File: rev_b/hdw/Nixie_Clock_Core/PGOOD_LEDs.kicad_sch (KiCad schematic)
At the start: 17 parts

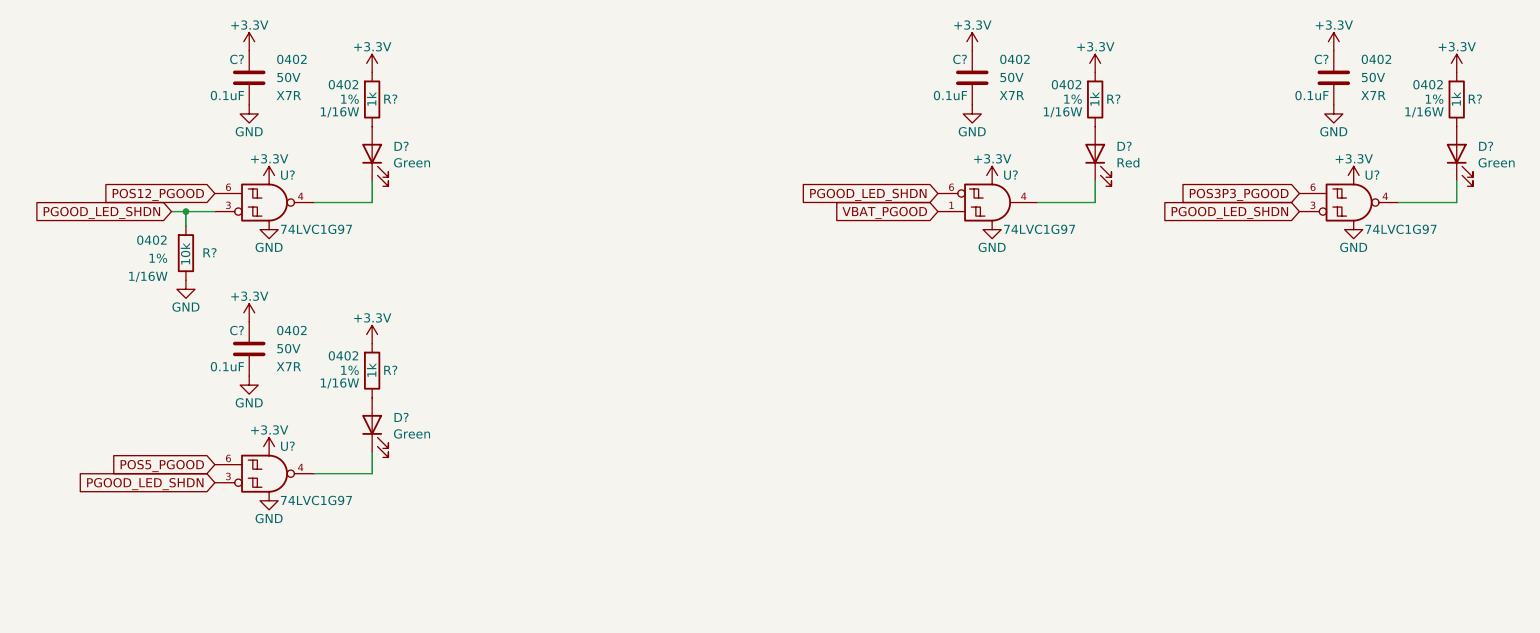
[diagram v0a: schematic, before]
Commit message: more carrier board progress
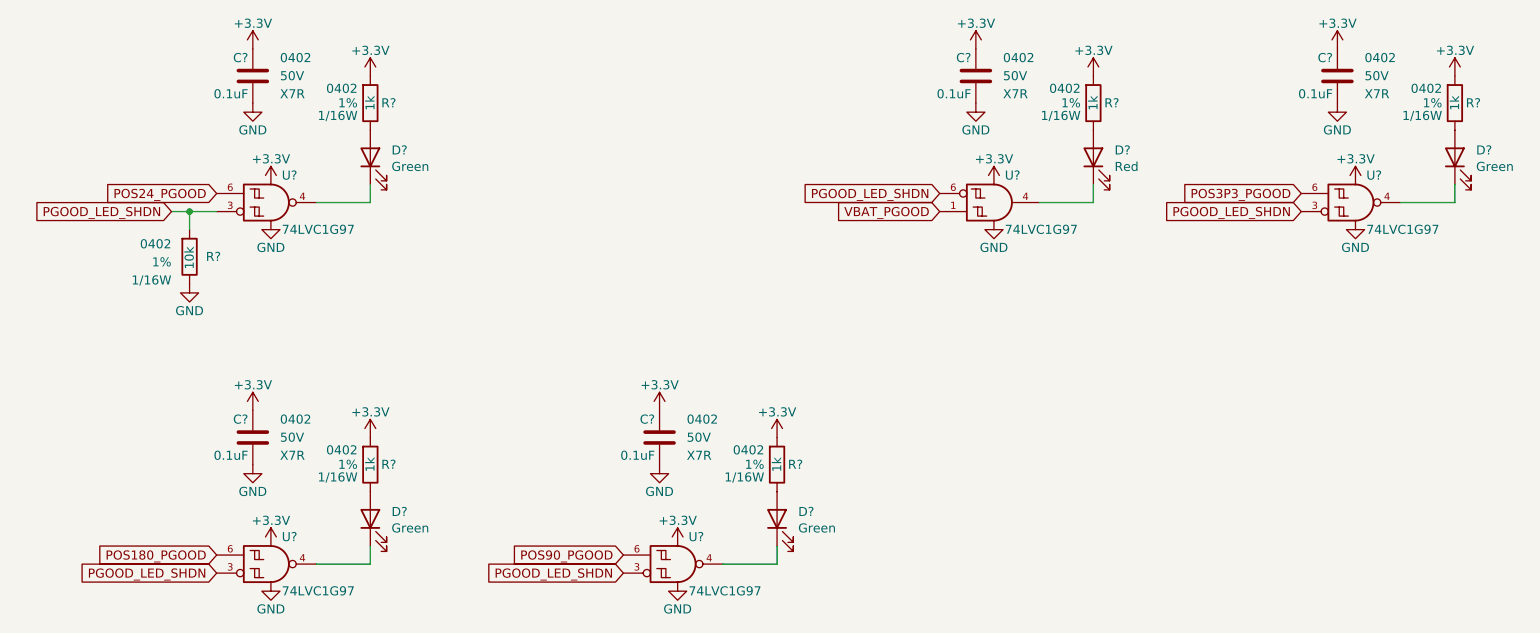
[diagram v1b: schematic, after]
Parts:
- added C?: 0.1uF, Capacitors_SMD:C_0402, symbol Custom_Library:C_Custom
- added D?: Green, LEDs:LED_0402, symbol Device:LED
- added R?: 1k, Resistors_SMD:R_0402, symbol Custom_Library:R_Custom
- added U?: 74LVC1G97, Package_TO_SOT_SMD:SOT-363_SC-70-6, symbol Custom_Library:74LVC1G97_Power_NAND_INV
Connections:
- net +3.3V: now also C?.1, R?.1, U?.1 (VCC), U?.5 (VCC)
- net GND: now also C?.2, U?.2 (GND)
- net PGOOD_LED_SHDN: now also U?.3
- net POS12_PGOOD renamed POS24_PGOOD
- net POS5_PGOOD renamed POS180_PGOOD
- new net: D?.1 (K), U?.4
- new net: D?.2 (A), R?.2
- new net POS90_PGOOD: U?.6
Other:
- moved on the sheet: C?, D?, R?, U?
